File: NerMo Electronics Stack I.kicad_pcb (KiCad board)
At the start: 2 copper layers, 83 x 66.4 mm, 80 parts, among them J1 PWM 5, J10 PWM 8, J11 PWM 9, J12 PWM 10, J13 PWM 11, J14 PWM 12, J15 PWM 13, J16 PWM 14, J17 PWM 15, J18 PWM 16, J2 Raspberry_Pi_Zero, J20 VBAT_IN, J3 PWM 1, J4 Address_Sel, J5 PWM 2, J6 PWM 3, J7 PWM 4, J8 PWM 6, J9 PWM 7, Q1 IRF7404, SW1 SW_SPDT, U3 AMS1117-3.3, U5 PCA9685PW, U6 INA3221

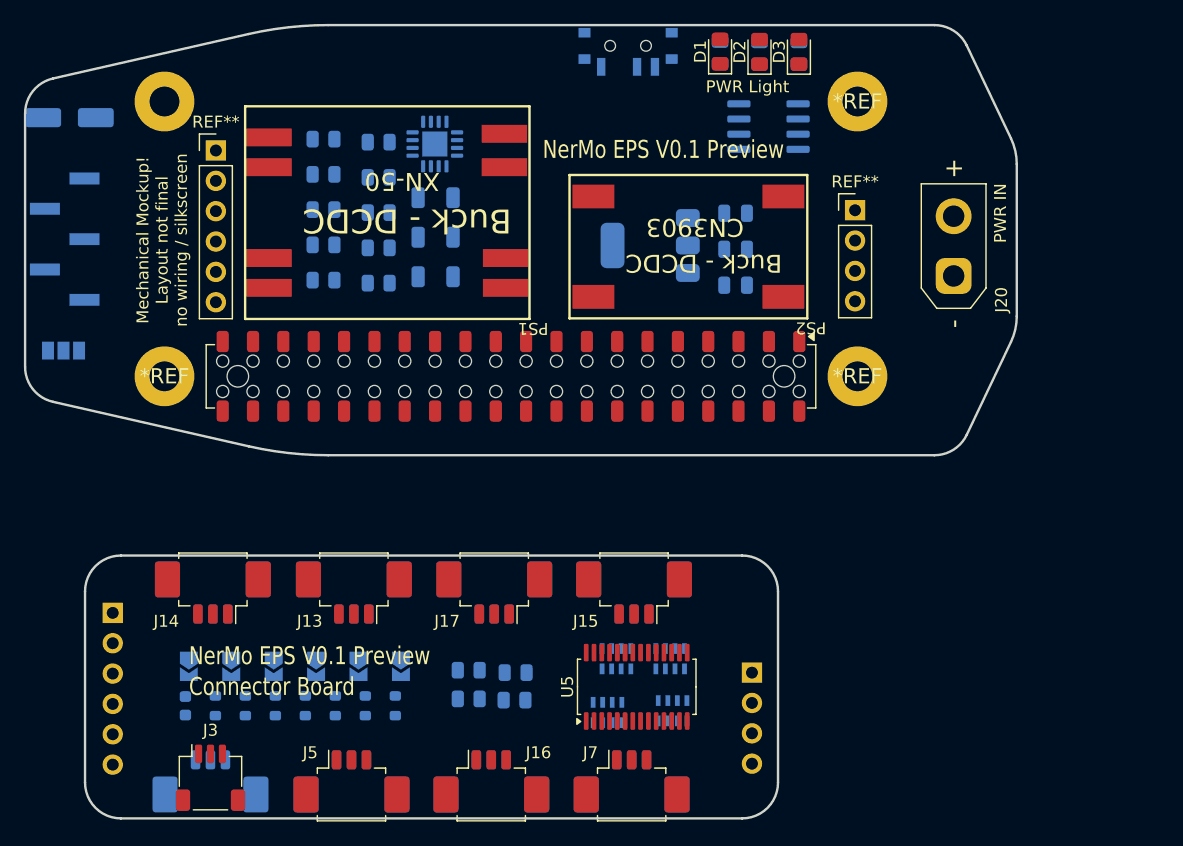
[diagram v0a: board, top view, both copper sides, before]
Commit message: feat: NerMo Stack V1
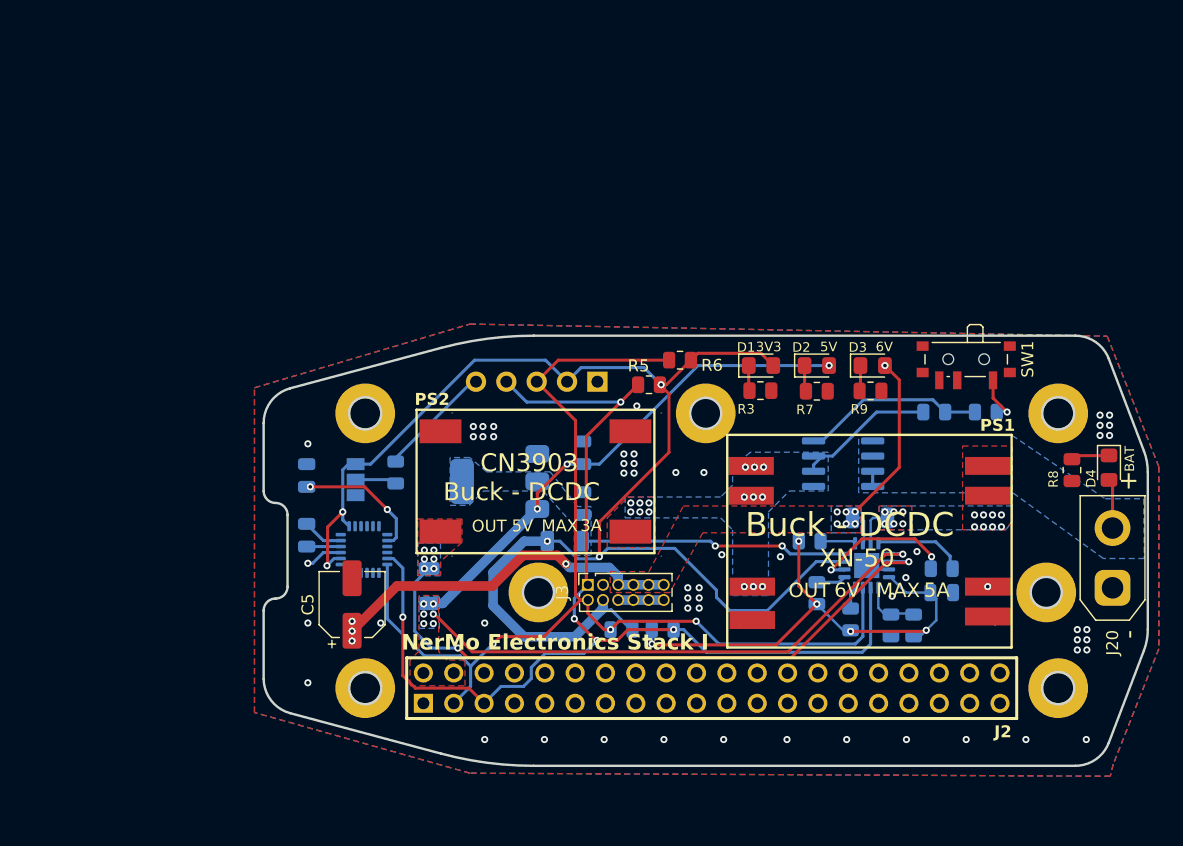
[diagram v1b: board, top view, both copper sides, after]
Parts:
- removed the *REF at (112.7, 85.4)
- removed the *REF at (112.7, 62.4)
- removed the *REF at (54.7, 85.4)
- removed C4: 10uF, Capacitor_SMD:C_0603_1608Metric
- removed J1: PWM 5, Connector_Molex:Molex_PicoBlade_53261-0371_1x03-1MP_P1.25mm_Horizontal
- removed J10: PWM 8, Connector_Molex:Molex_PicoBlade_53261-0371_1x03-1MP_P1.25mm_Horizontal
- removed J11: PWM 9, Connector_Molex:Molex_PicoBlade_53261-0371_1x03-1MP_P1.25mm_Horizontal
- removed J12: PWM 10, Connector_Molex:Molex_PicoBlade_53261-0371_1x03-1MP_P1.25mm_Horizontal
- removed J13: PWM 11, Connector_Molex:Molex_PicoBlade_53261-0371_1x03-1MP_P1.25mm_Horizontal
- removed J14: PWM 12, Connector_Molex:Molex_PicoBlade_53261-0371_1x03-1MP_P1.25mm_Horizontal
- removed J15: PWM 13, Connector_Molex:Molex_PicoBlade_53261-0371_1x03-1MP_P1.25mm_Horizontal
- removed J16: PWM 14, Connector_Molex:Molex_PicoBlade_53261-0371_1x03-1MP_P1.25mm_Horizontal
- removed J17: PWM 15, Connector_Molex:Molex_PicoBlade_53261-0371_1x03-1MP_P1.25mm_Horizontal
- removed J18: PWM 16, Connector_Molex:Molex_PicoBlade_53261-0371_1x03-1MP_P1.25mm_Horizontal
- removed J5: PWM 2, Connector_Molex:Molex_PicoBlade_53261-0371_1x03-1MP_P1.25mm_Horizontal
- removed J6: PWM 3, Connector_Molex:Molex_PicoBlade_53261-0371_1x03-1MP_P1.25mm_Horizontal
- removed J7: PWM 4, Connector_Molex:Molex_PicoBlade_53261-0371_1x03-1MP_P1.25mm_Horizontal
- removed J8: PWM 6, Connector_Molex:Molex_PicoBlade_53261-0371_1x03-1MP_P1.25mm_Horizontal
- removed J9: PWM 7, Connector_Molex:Molex_PicoBlade_53261-0371_1x03-1MP_P1.25mm_Horizontal
- removed JP3: Addr0, Jumper:SolderJumper-2_P1.3mm_Open_TrianglePad1.0x1.5mm
- removed JP4: Addr1, Jumper:SolderJumper-2_P1.3mm_Open_TrianglePad1.0x1.5mm
- removed JP5: Addr2, Jumper:SolderJumper-2_P1.3mm_Open_TrianglePad1.0x1.5mm
- removed JP6: Addr3, Jumper:SolderJumper-2_P1.3mm_Open_TrianglePad1.0x1.5mm
- removed JP7: Addr4, Jumper:SolderJumper-2_P1.3mm_Open_TrianglePad1.0x1.5mm
- removed JP8: Addr5, Jumper:SolderJumper-2_P1.3mm_Open_TrianglePad1.0x1.5mm
- removed R11: 4k7, Resistor_SMD:R_0805_2012Metric
- removed R12, R13, R14, R15, R16, R17, R18: 10k, Resistor_SMD:R_0603_1608Metric
- removed REF**: PinHeader_1x04_P2.54mm_Vertical, Connector_PinHeader_2.54mm:PinHeader_1x04_P2.54mm_Vertical
- removed REF**: PinHeader_1x06_P2.54mm_Vertical, Connector_PinHeader_2.54mm:PinHeader_1x06_P2.54mm_Vertical
- removed REF**: MountingHole_2.5mm_Pad, MountingHole:MountingHole_2.5mm_Pad
- removed REF**: PinSocket_1x04_P2.54mm_Vertical, Connector_PinSocket_2.54mm:PinSocket_1x04_P2.54mm_Vertical
- removed REF**: PinSocket_1x06_P2.54mm_Vertical, Connector_PinSocket_2.54mm:PinSocket_1x06_P2.54mm_Vertical
- removed RN1, RN2, RN3, RN4: 220, Resistor_SMD:R_Array_Concave_4x0603
- removed U5: PCA9685PW, Package_SO:TSSOP-28_4.4x9.7mm_P0.65mm
- added *REF: , , F.Cu at (100.0, 88.5)
- added *REF: , , F.Cu at (86.0, 103.5)
- added *REF: , , F.Cu at (71.5, 88.5)
- added *REF: , , F.Cu at (129.5, 111.5)
- added *REF: , , F.Cu at (129.5, 88.5)
- added *REF: , , F.Cu at (71.5, 111.5)
- added *REF: , , F.Cu at (128.5, 103.5)
- added C1: 2.2uF, Capacitor_SMD:C_0805_2012Metric, B.Cu at (66.6, 93.7)
- added C2: 0.1uF, Capacitor_SMD:C_0805_2012Metric, B.Cu at (66.6, 98.7)
- added D4: LED, LED_SMD:LED_0805_2012Metric_Pad1.15x1.40mm_HandSolder, F.Cu at (133.8, 93.0)
- added R8: 3k, Resistor_SMD:R_0805_2012Metric, F.Cu at (130.7, 93.2)
- added U1: MPU-6050, Sensor_Motion:InvenSense_QFN-24_4x4mm_P0.5mm, B.Cu at (71.4, 99.9)
- C5, R3, R5, R6, R7, R9, SW1: moved to F.Cu
- J2: footprint Custom_Modules:Raspberry_Pi_Zero_2_W_Underside_LowProfile -> Custom_Modules:Raspberry_Pi_Zero_2_W_HDR-TH
- J3: value PWM 1 -> Conn_02x06_Odd_Even; footprint Connector_JST:JST_SH_SM03B-SRSS-TB_1x03-1MP_P1.00mm_Horizontal -> Connector_PinSocket_1.27mm:PinSocket_2x06_P1.27mm_Vertical
- U2: footprint Connector_PinHeader_2.54mm:PinHeader_1x05_P2.54mm_Vertical_SMD_Pin1Left -> Connector_PinHeader_2.54mm:PinHeader_1x05_P2.54mm_Vertical
- moved R38 60.4 mm to (117.4, 106.2), turned to 90 degrees
- moved R1 60.0 mm to (123.4, 88.4)
- moved R39 58.4 mm to (119.8, 101.5)
- moved R43 55.1 mm to (115.5, 106.2), turned to -90 degrees
- moved R2 54.8 mm to (119.1, 88.4)
- moved R40 52.5 mm to (112.1, 105.8), turned to -90 degrees
- moved U6 50.5 mm to (113.5, 101.2)
- moved C5 47.1 mm to (70.4, 104.5), turned to 90 degrees
- moved R44 46.7 mm to (109.3, 103.5), turned to -90 degrees
- moved U2 46.2 mm to (90.9, 85.9), turned to 90 degrees
- moved R41 45.6 mm to (93.0, 106.6), turned to 0 degrees
- moved R42 44.7 mm to (96.4, 106.6)
- moved R36 43.3 mm to (113.8, 97.2), turned to 0 degrees
- moved R45 42.0 mm to (108.7, 99.2)
- moved SW1 38.6 mm to (121.8, 84.3), turned to 180 degrees
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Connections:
- C5 pad 1: +3.3V -> +6V
- J20 pad 1: BAT_GND -> GND
- J3 pad 1: Net-(J3-Pin_1) -> /I2C_SCL
- J3 pad 2: +6V -> /I2C_SDA
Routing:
- net +3.3V: track 0.00 -> 168.3 mm, vias 0 -> 10
- net /I2C_SCL: track 0.00 -> 94.5 mm, vias 0 -> 5
- net /I2C_SDA: track 0.00 -> 90.7 mm, vias 0 -> 3
- net +5V: track 0.00 -> 87.6 mm, vias 0 -> 10
- net +5V_PWR: track 0.00 -> 53.0 mm, vias 0 -> 8
- net +6V: track 0.00 -> 47.4 mm, vias 0 -> 11
- net +3.3V_PWR: track 0.00 -> 22.4 mm, vias 0 -> 2
- net Net-(Q1-G): track 0.00 -> 15.4 mm
- net GND: track 0.00 -> 12.4 mm, vias 0 -> 56
- net Net-(U6-PV): track 0.00 -> 12.3 mm, vias 0 -> 2
- net VBAT: track 0.00 -> 11.6 mm, vias 0 -> 15
- net Net-(U1-CPOUT): track 0.00 -> 10.8 mm, vias 0 -> 2
- net /IMU1_I2C_Sel: track 0.00 -> 10.1 mm
- net Net-(U6-VPU): track 0.00 -> 7.56 mm
- net VBAT_IN: track 0.00 -> 5.42 mm
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- added copper zone on B.Cu, net +3.3V_PWR
- added copper zone on B.Cu, net +5V
- added copper zone on F.Cu, net +5V
- added copper zone on B.Cu, net +5V_PWR
- added copper zone on F.Cu, net +5V_PWR
- added copper zone on B.Cu, net +6V
- added copper zone on F.Cu, net +6V
- added copper zone on B.Cu, net +6V_PWR
- added copper zone on F.Cu, net +6V_PWR
- added copper zone on B.Cu, net GND
- added copper zone on F.Cu, net GND
- added copper zone on B.Cu, net VBAT
- added copper zone on F.Cu, net VBAT
- added copper zone on B.Cu, net VBAT_IN
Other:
- board size 83 x 66.4 mm -> 74 x 36 mm
- board text added: "3A"
- board text added: "3V3"
- board text added: "3V3 1A LDO"
- board text added: "5A"
- board text added: "5V"
- board text added: "6V"
- board text added: "BAT"
- board text added: "INA3221 PMON"
- board text added: "MAX"
- board text added: "NerMo Electronics Stack I"
- board text added: "OUT"
- board text removed: "Connector Board"
- board text removed: "Mechanical Mockup! Layout not final no wiring / silkscreen"
- board text removed: "NerMo EPS V0.1 Preview"
- board text removed: "PWR IN"
- board text removed: "PWR Light"
- board text removed: "Tail"
